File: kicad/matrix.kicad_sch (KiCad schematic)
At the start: 72 parts, among them SW401 SW_Push_Dual, SW402 SW_Push_Dual, SW403 SW_Push_Dual, SW404 SW_Push_Dual, SW405 SW_Push_Dual, SW406 SW_Push_Dual, SW407 SW_Push_Dual, SW408 SW_Push_Dual, SW409 SW_Push_Dual, SW410 SW_Push_Dual, SW411 SW_Push_Dual, SW412 SW_Push_Dual, SW413 SW_Push_Dual, SW414 SW_Push_Dual, SW415 SW_Push_Dual, SW416 SW_Push_Dual, SW417 SW_Push_Dual, SW418 SW_Push_Dual, SW419 SW_Push_Dual, SW420 SW_Push_Dual, SW421 SW_Push_Dual, SW422 SW_Push_Dual, SW423 SW_Push_Dual, SW424 SW_Push_Dual, SW425 SW_Push_Dual, SW426 SW_Push_Dual, SW427 SW_Push_Dual, SW428 SW_Push_Dual, SW429 SW_Push_Dual, SW430 SW_Push_Dual, SW431 SW_Push_Dual, SW432 SW_Push_Dual, SW433 SW_Push_Dual, SW434 SW_Push_Dual, SW435 SW_Push_Dual, SW436 SW_Push_Dual

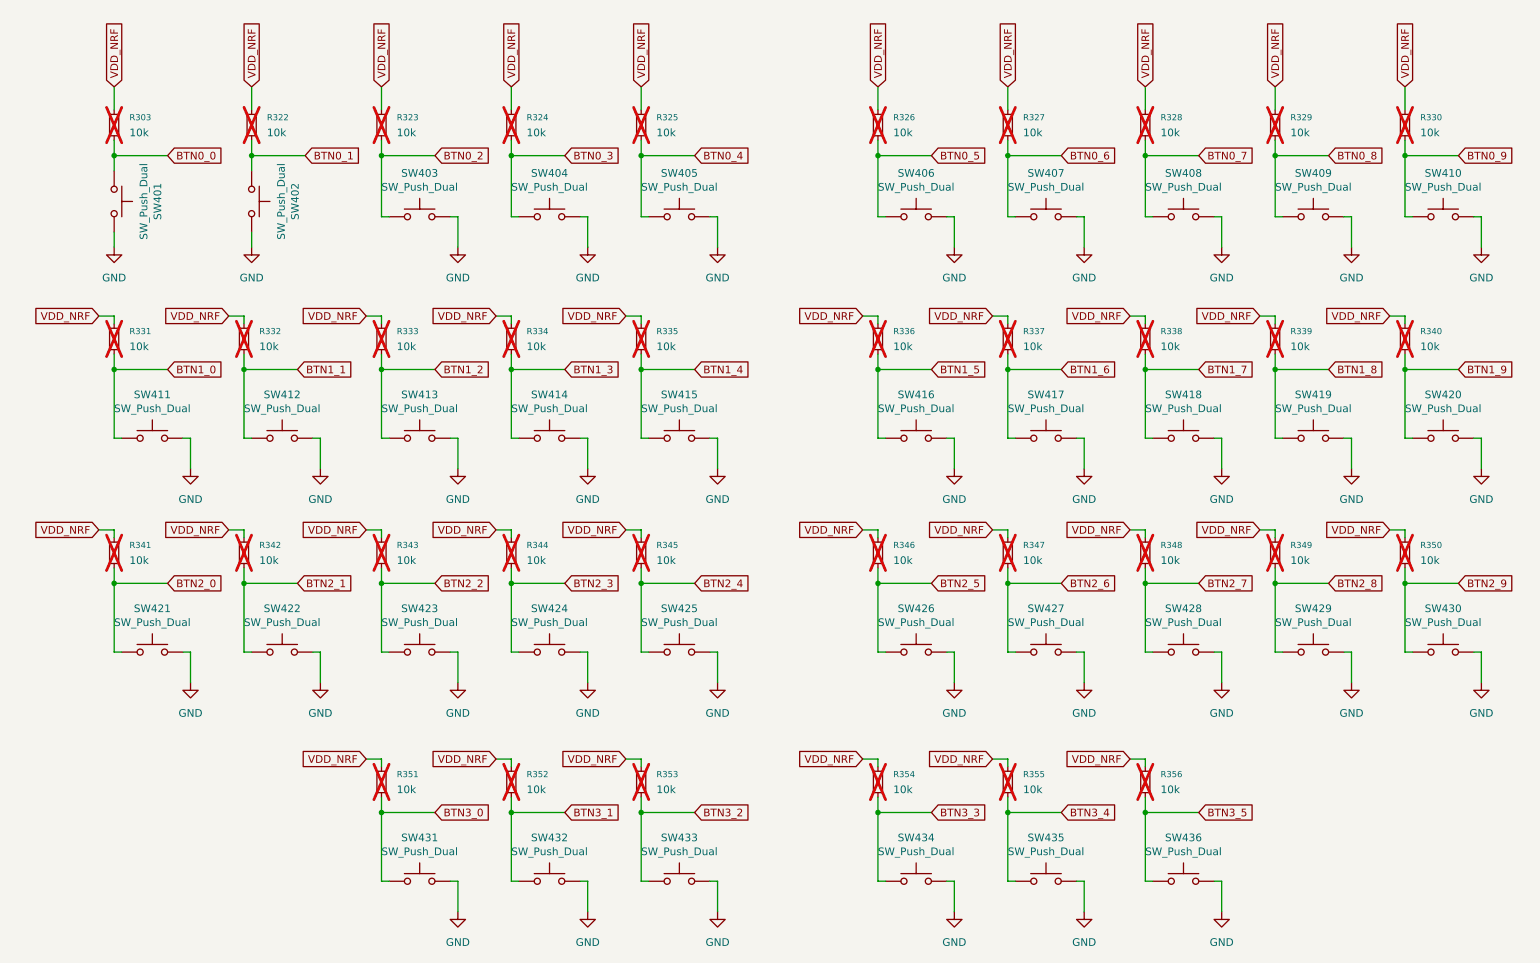
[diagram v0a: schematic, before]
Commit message: board routed
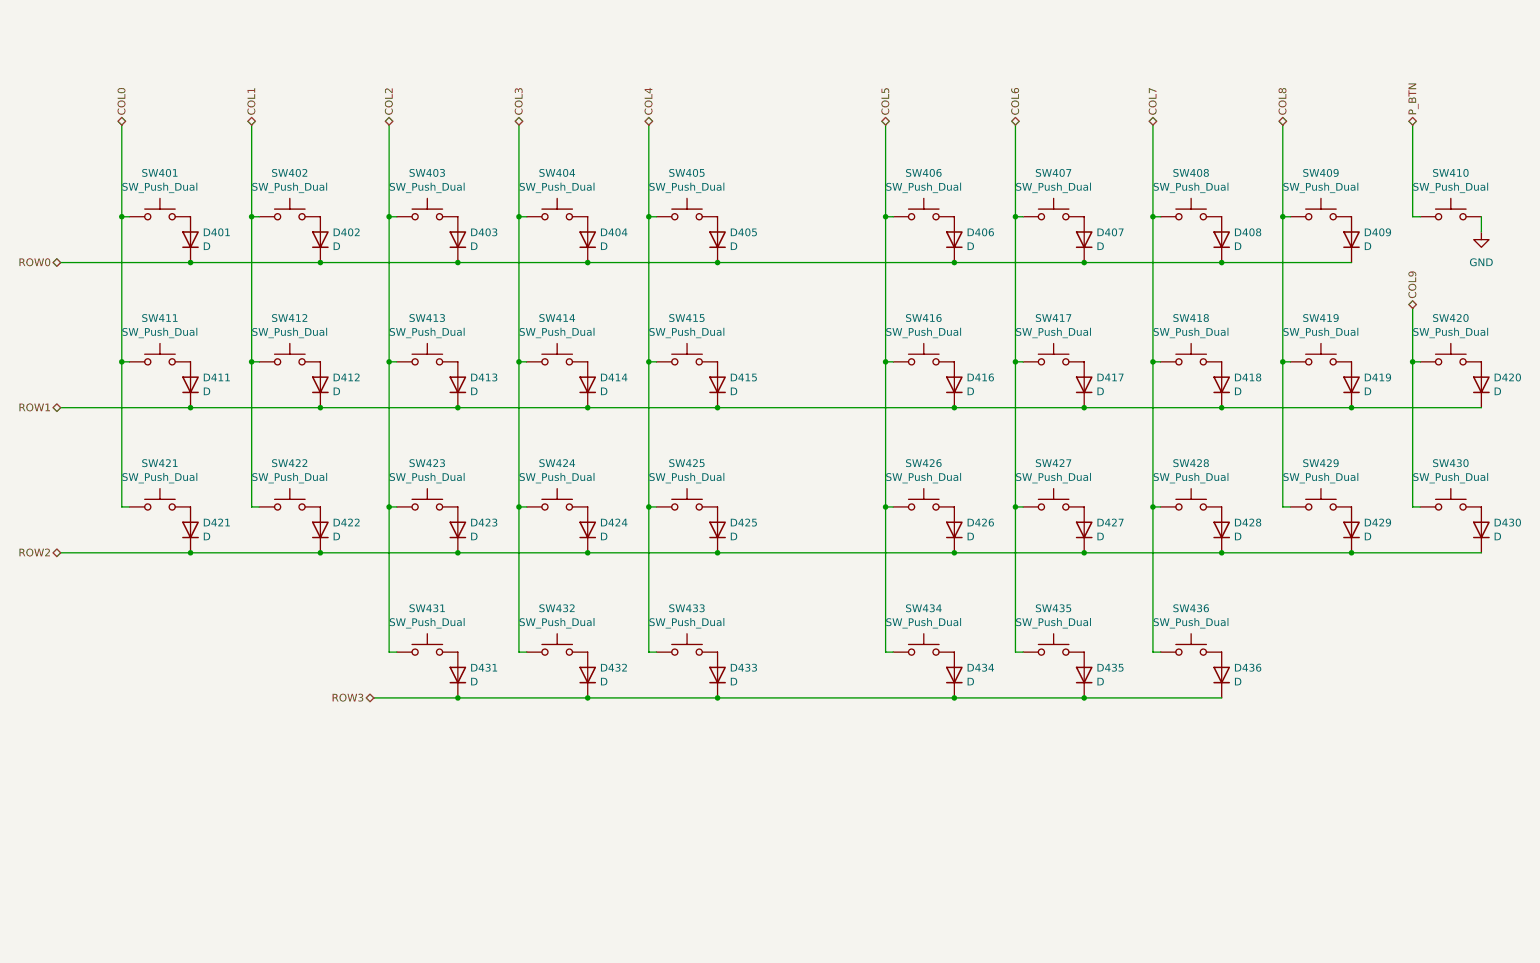
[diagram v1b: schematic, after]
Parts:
- removed R303, R322, R323, R324, R325, R326, R327, R328, R329, R330, R331, R332, R333, R334, R335, R336, R337, R338, R339, R340, R341, R342, R343, R344, R345, R346, R347, R348, R349, R350, R351, R352, R353, R354, R355, R356: 10k, Resistor_SMD:R_0603_1608Metric, symbol Device:R_Small
- added D401, D402, D403, D404, D405, D406, D407, D408, D409, D411, D412, D413, D414, D415, D416, D417, D418, D419, D420, D421, D422, D423, D424, D425, D426, D427, D428, D429, D430, D431, D432, D433, D434, D435, D436: D, Diode_SMD:D_SOD-123, symbol Device:D
- SW401, SW402, SW403, SW404, SW405, SW406, SW407, SW408, SW409, SW410, SW411, SW412, SW413, SW414, SW415, SW416, SW417, SW418, SW419, SW420, SW421, SW422, SW423, SW424, SW425, SW426, SW427, SW428, SW429, SW430, SW431, SW432, SW433, SW434, SW435, SW436: footprint Button_Switch_THT:SW_PUSH_6mm_H7.3mm -> Button_Switch_THT:SW_PUSH_6mm
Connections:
- net BTN1_0 is gone; now on net COL0: SW411.1
- net BTN1_1 is gone; now on net COL1: SW412.1
- net BTN1_2 is gone; now on net COL2: SW413.1
- net BTN1_3 is gone; now on net COL3: SW414.1
- net BTN1_4 is gone; now on net COL4: SW415.1
- net BTN1_5 is gone; now on net COL5: SW416.1
- net BTN1_6 is gone; now on net COL6: SW417.1
- net BTN1_7 is gone; now on net COL7: SW418.1
- net BTN1_8 is gone; now on net COL8: SW419.1
- net BTN2_0 is gone; now on net COL0: SW421.1
- net BTN2_1 is gone; now on net COL1: SW422.1
- net BTN2_2 is gone; now on net COL2: SW423.1
- net BTN2_3 is gone; now on net COL3: SW424.1
- net BTN2_4 is gone; now on net COL4: SW425.1
- net BTN2_5 is gone; now on net COL5: SW426.1
- net BTN2_6 is gone; now on net COL6: SW427.1
- net BTN2_7 is gone; now on net COL7: SW428.1
- net BTN2_8 is gone; now on net COL8: SW429.1
- net BTN2_9 is gone; now on net COL9: SW430.1
- net BTN3_0 is gone; now on net COL2: SW431.1
- net BTN3_1 is gone; now on net COL3: SW432.1
- net BTN3_2 is gone; now on net COL4: SW433.1
- net BTN3_3 is gone; now on net COL5: SW434.1
- net BTN3_4 is gone; now on net COL6: SW435.1
- net BTN3_5 is gone; now on net COL7: SW436.1
- net GND: no longer SW401.2, SW402.2, SW403.2, SW404.2, SW405.2, SW406.2, SW407.2, SW408.2, SW409.2, SW411.2, SW412.2, SW413.2, SW414.2, SW415.2, SW416.2, SW417.2, SW418.2, SW419.2, SW420.2, SW421.2, SW422.2, SW423.2, SW424.2, SW425.2, SW426.2, SW427.2, SW428.2, SW429.2, SW430.2, SW431.2, SW432.2, SW433.2, SW434.2, SW435.2, SW436.2
- net BTN0_0 renamed COL0
- net BTN0_1 renamed COL1
- net BTN0_2 renamed COL2
- net BTN0_3 renamed COL3
- net BTN0_4 renamed COL4
- net BTN0_5 renamed COL5
- net BTN0_6 renamed COL6
- net BTN0_7 renamed COL7
- net BTN0_8 renamed COL8
- net BTN0_9 renamed P_BTN
- net BTN1_9 renamed COL9
- new net: D404.2 (A), SW404.2
- new net: D401.2 (A), SW401.2
- new net: D425.2 (A), SW425.2
- new net: D408.2 (A), SW408.2
- new net: D405.2 (A), SW405.2
- new net: D422.2 (A), SW422.2
- new net: D426.2 (A), SW426.2
- new net: D414.2 (A), SW414.2
- new net: D434.2 (A), SW434.2
- new net: D436.2 (A), SW436.2
- new net: D412.2 (A), SW412.2
- new net: D428.2 (A), SW428.2
- new net: D403.2 (A), SW403.2
- new net: D424.2 (A), SW424.2
- new net: D416.2 (A), SW416.2
- new net: D435.2 (A), SW435.2
- new net: D402.2 (A), SW402.2
- new net: D420.2 (A), SW420.2
- new net: D430.2 (A), SW430.2
- new net: D415.2 (A), SW415.2
- new net: D419.2 (A), SW419.2
- new net: D433.2 (A), SW433.2
- new net: D417.2 (A), SW417.2
- new net: D432.2 (A), SW432.2
- new net: D411.2 (A), SW411.2
- new net: D429.2 (A), SW429.2
- new net: D407.2 (A), SW407.2
- new net: D418.2 (A), SW418.2
- new net: D431.2 (A), SW431.2
- new net: D409.2 (A), SW409.2
- new net: D413.2 (A), SW413.2
- new net: D427.2 (A), SW427.2
- new net: D423.2 (A), SW423.2
- new net: D406.2 (A), SW406.2
- new net: D421.2 (A), SW421.2
- new net ROW0: D401.1 (K), D402.1 (K), D403.1 (K), D404.1 (K), D405.1 (K), D406.1 (K), D407.1 (K), D408.1 (K), D409.1 (K)
- new net ROW1: D411.1 (K), D412.1 (K), D413.1 (K), D414.1 (K), D415.1 (K), D416.1 (K), D417.1 (K), D418.1 (K), D419.1 (K), D420.1 (K)
- new net ROW2: D421.1 (K), D422.1 (K), D423.1 (K), D424.1 (K), D425.1 (K), D426.1 (K), D427.1 (K), D428.1 (K), D429.1 (K), D430.1 (K)
- new net ROW3: D431.1 (K), D432.1 (K), D433.1 (K), D434.1 (K), D435.1 (K), D436.1 (K)
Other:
- moved on the sheet: SW401, SW402, SW403, SW404, SW405, SW406, SW407, SW408, SW409, SW410, SW411, SW412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
